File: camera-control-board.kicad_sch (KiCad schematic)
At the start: 51 parts, among them J1 DF12NB-36DS-0.5V_51_, J2 10104110-0001LF, J3 104031-0811, J4 02x05 M 1.27mm, J5 Conn_01x08, SW1 CAS-120TA, SW3 SW_Push, U1 STM32H743IITx, U2 IS42S32800J-7TLI, U3 W25Q256JVEIQ TR, U4 XC6210B332MR, Y1 12MHz/7pF

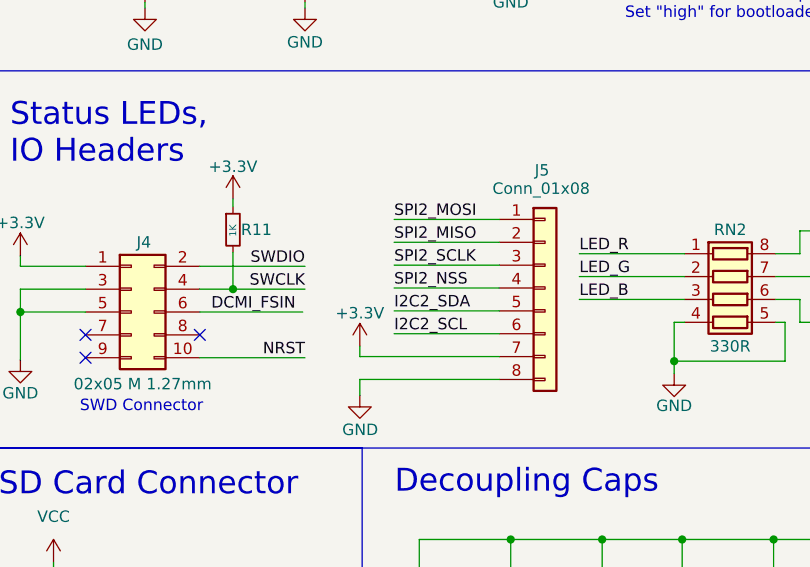
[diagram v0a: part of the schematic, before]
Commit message: Layout begun.
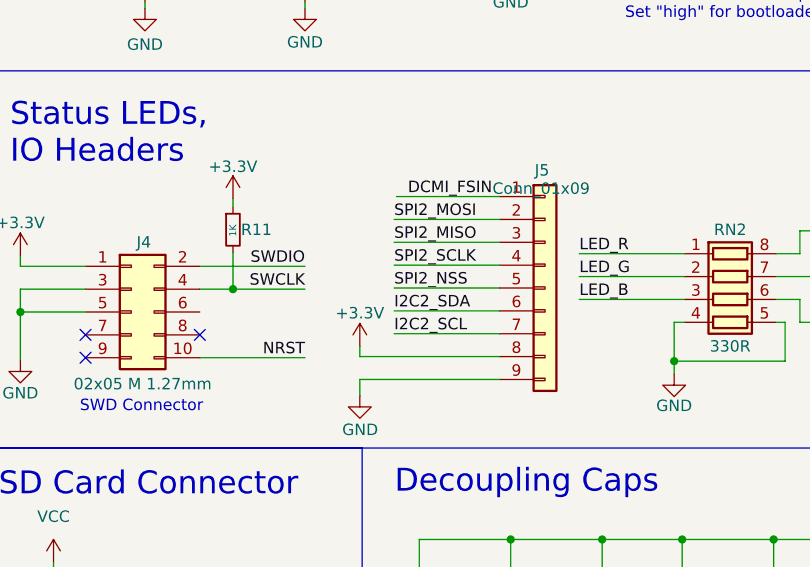
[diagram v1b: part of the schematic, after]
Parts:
- J5: value Conn_01x08 -> Conn_01x09; footprint Connector_PinHeader_2.54mm:PinHeader_1x08_P2.54mm_Vertical -> Connector_PinHeader_2.54mm:PinHeader_1x09_P2.54mm_Vertical; symbol Connector_Generic:Conn_01x08 -> Connector_Generic:Conn_01x09
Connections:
- net +3.3V: now also J5.8 (Pin_8); no longer J5.7 (Pin_7)
- net DCMI_FSIN: now also J5.1 (Pin_1); no longer J4.6 (Pin_6)
- net GND: now also J5.9 (Pin_9); no longer J5.8 (Pin_8)
- net I2C2_SCL: now also J5.7 (Pin_7); no longer J5.6 (Pin_6)
- net I2C2_SDA: now also J5.6 (Pin_6); no longer J5.5 (Pin_5)
- net SPI2_MISO: now also J5.3 (Pin_3); no longer J5.2 (Pin_2)
- net SPI2_MOSI: now also J5.2 (Pin_2); no longer J5.1 (Pin_1)
- net SPI2_NSS: now also J5.5 (Pin_5); no longer J5.4 (Pin_4)
- net SPI2_SCLK: now also J5.4 (Pin_4); no longer J5.3 (Pin_3)
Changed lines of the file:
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@@
 	(wire
 		(pts
+			(xy 198.12 100.33) (xy 209.55 100.33)
+		)
+		(stroke
+			(width 0)
+			(type default)
+		)
+	)
+	(wire
+		(pts
 			(xy 352.806 106.68) (xy 352.806 111.76)
 		)
@@
 	(wire
 		(pts
-			(xy 176.276 113.157) (xy 187.706 113.157)
-		)
-		(stroke
-			(width 0)
-			(type default)
-		)
-	)
-	(wire
-		(pts
 			(xy 34.29 73.66) (xy 46.99 73.66)
 		)
@@
 		)
 	)
+	(label "DCMI_FSIN"
+		(at 199.39 100.33 0)
+		(fields_autoplaced yes)
+		(effects
+			(font
+				(size 1.27 1.27)
+			)
+			(justify left bottom)
+		)
+	)
 	(label "I2C2_SDA"
 		(at 197.866 113.03 0)
@@
 		)
 	)
-	(label "DCMI_FSIN"
-		(at 177.546 113.157 0)
-		(fields_autoplaced yes)
-		(effects
-			(font
-				(size 1.27 1.27)
-			)
-			(justify left bottom)
-		)
-	)
 	(label "DRAM_D19"
 		(at 38.1 132.08 0)
@@
 	)
 	(symbol
-		(lib_id "Connector_Generic:Conn_01x08")
+		(lib_id "Connector_Generic:Conn_01x09")
 		(at 214.63 110.49 0)
 		(unit 1)
 		(exclude_from_sim no)
 		(in_bom yes)
-		(on_board no)
+		(on_board yes)
 		(dnp no)
 		(property "Reference" "J5"
@@
 			)
 		)
-		(property "Value" "Conn_01x08"
+		(property "Value" "Conn_01x09"
 			(at 208.788 99.441 0)
 			(effects
@@
 			)
 		)
-		(property "Footprint" "Connector_PinHeader_2.54mm:PinHeader_1x08_P2.54mm_Vertical"
+		(property "Footprint" "Connector_PinHeader_2.54mm:PinHeader_1x09_P2.54mm_Vertical"
 			(at 214.63 110.49 0)
 			(effects
@@
 			)
 		)
-		(property "Description" ""
+		(property "Description" "Generic connector, single row, 01x09, script generated (kicad-library-utils/schlib/autogen/connector/)"
 			(at 214.63 110.49 0)
 			(effects
@@
 		(pin "8"
 		)
+		(pin "9"
+		)
 		(instances
